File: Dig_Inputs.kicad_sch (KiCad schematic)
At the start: 31 parts, among them J11 Digital, U3 LTV-357T

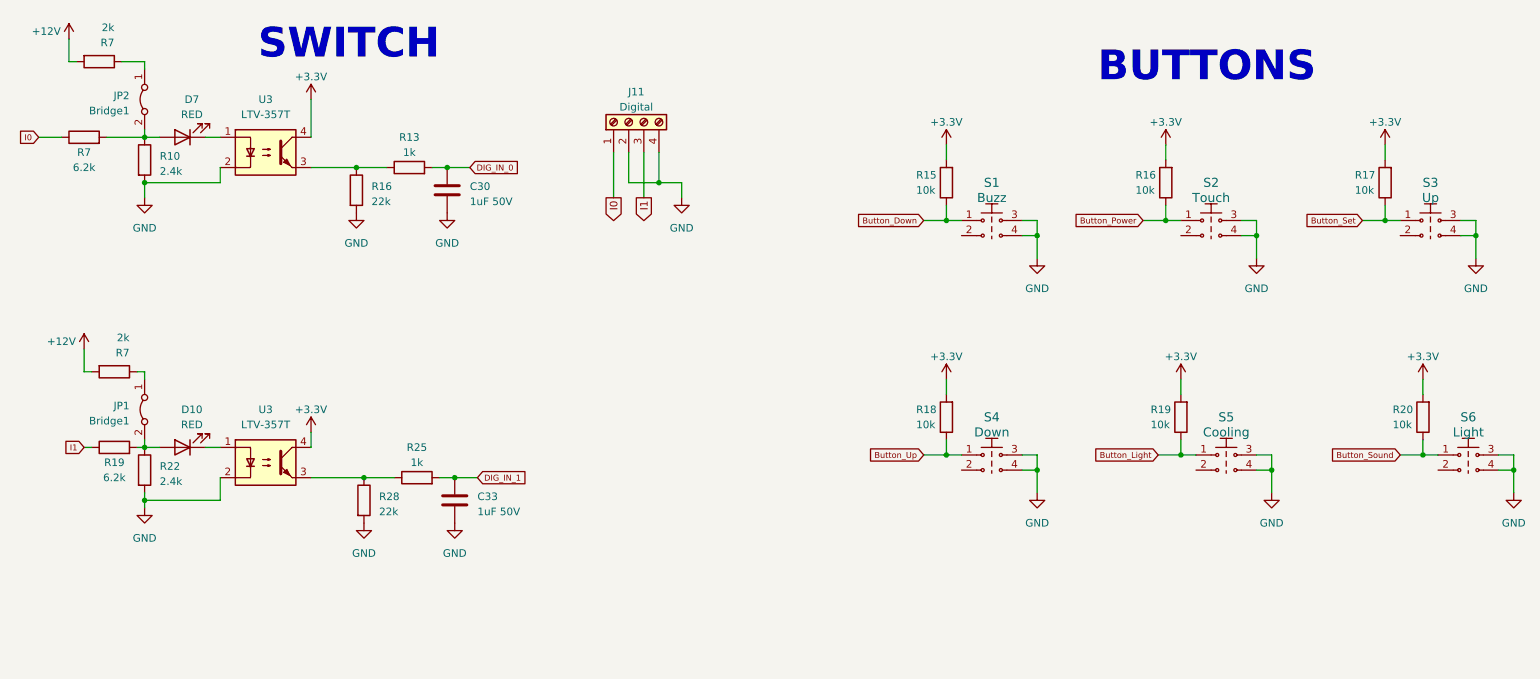
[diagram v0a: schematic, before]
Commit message: Luego de modificaciones de Dandy
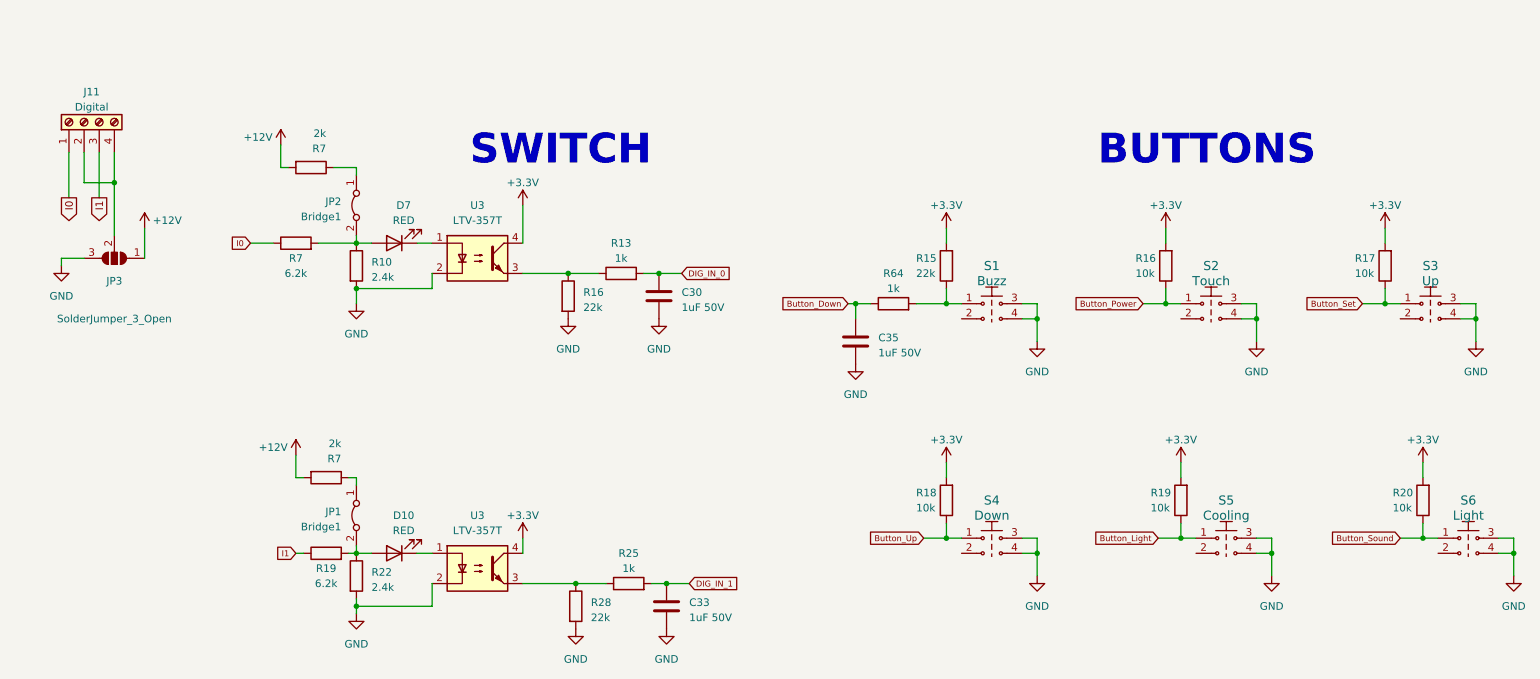
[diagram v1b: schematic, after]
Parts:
- added C35: 1uF 50V, 1-Capacitor:C_0805_2012Metric, symbol 1-Capacitor:C_0805
- added JP3: SolderJumper_3_Open, 1-Jumper:SolderJumper-3_P1.3mm_Open_RoundedPad1.0x1.5mm, symbol Jumper:SolderJumper_3_Open
- added R64: 1k, 1-Resistor:R_0805_2012Metric, symbol 1-Resistor:R_0805
- R15: value 10k -> 22k
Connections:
- net +12V: now also JP3.1 (A)
- net Button_Down: now also C35.1, R64.1; no longer R15.1, S1.1
- net GND: now also C35.2, JP3.3 (B); no longer J11.2 (Pin_2), J11.4 (Pin_4)
- new net: R15.1, R64.2, S1.1
- new net: J11.2 (Pin_2), J11.4 (Pin_4), JP3.2 (C)
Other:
- moved on the sheet: C30, C33, D10, D7, J11, JP1, JP2, R10, R13, R15, R16, R17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
